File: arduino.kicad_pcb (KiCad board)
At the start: 2 copper layers, 50.8 x 70.6 mm, 30 parts, among them J1 Conn_01x08_Pin, J10 Conn_01x06_Socket, J12 Conn_01x03_Pin, J2 Conn_01x10_Socket, J3 Barrel_Jack_Switch, J4 Conn_01x02_Socket, J5 Conn_01x06_Socket, J8 Conn_01x08_Pin, SW1 SW_Push, U1 ATmega328-P, U2 L7805, U3 LM317_TO-220, Y1 Crystal

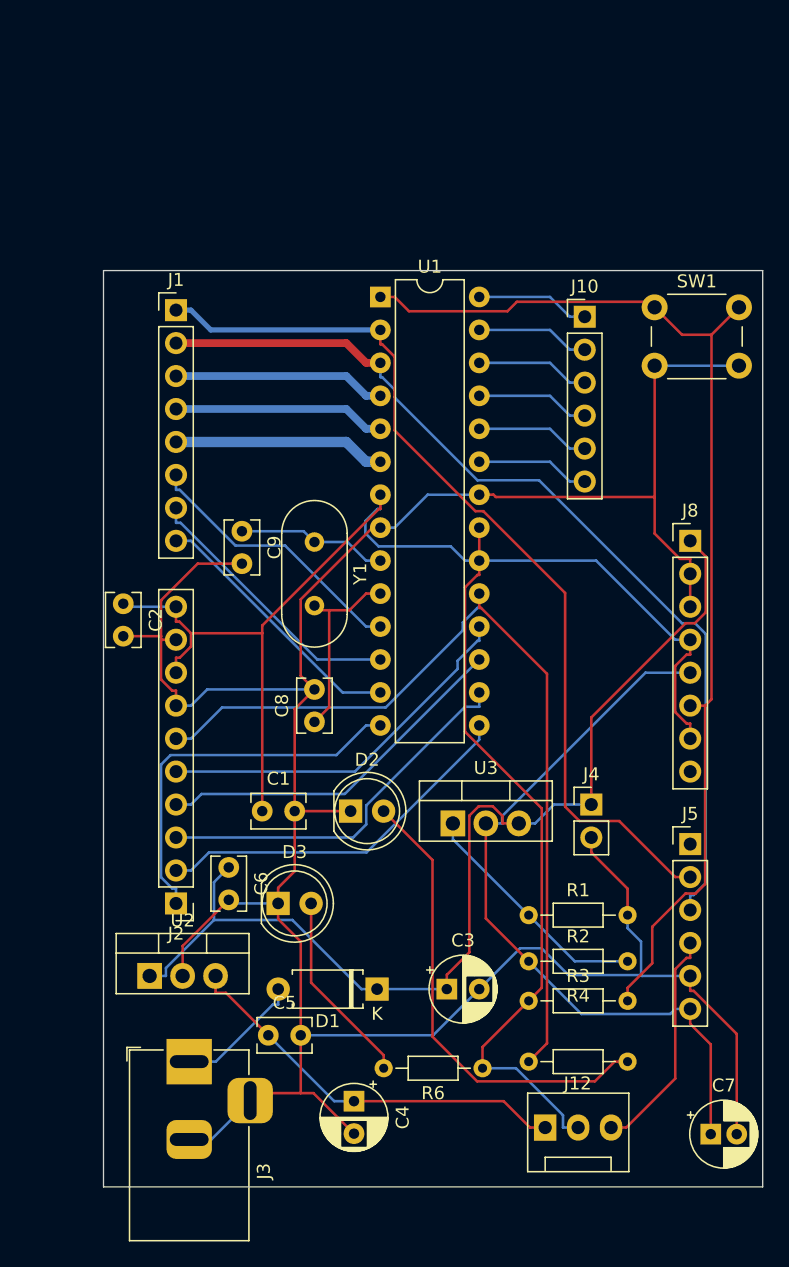
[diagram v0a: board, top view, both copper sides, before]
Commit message: Add files via upload
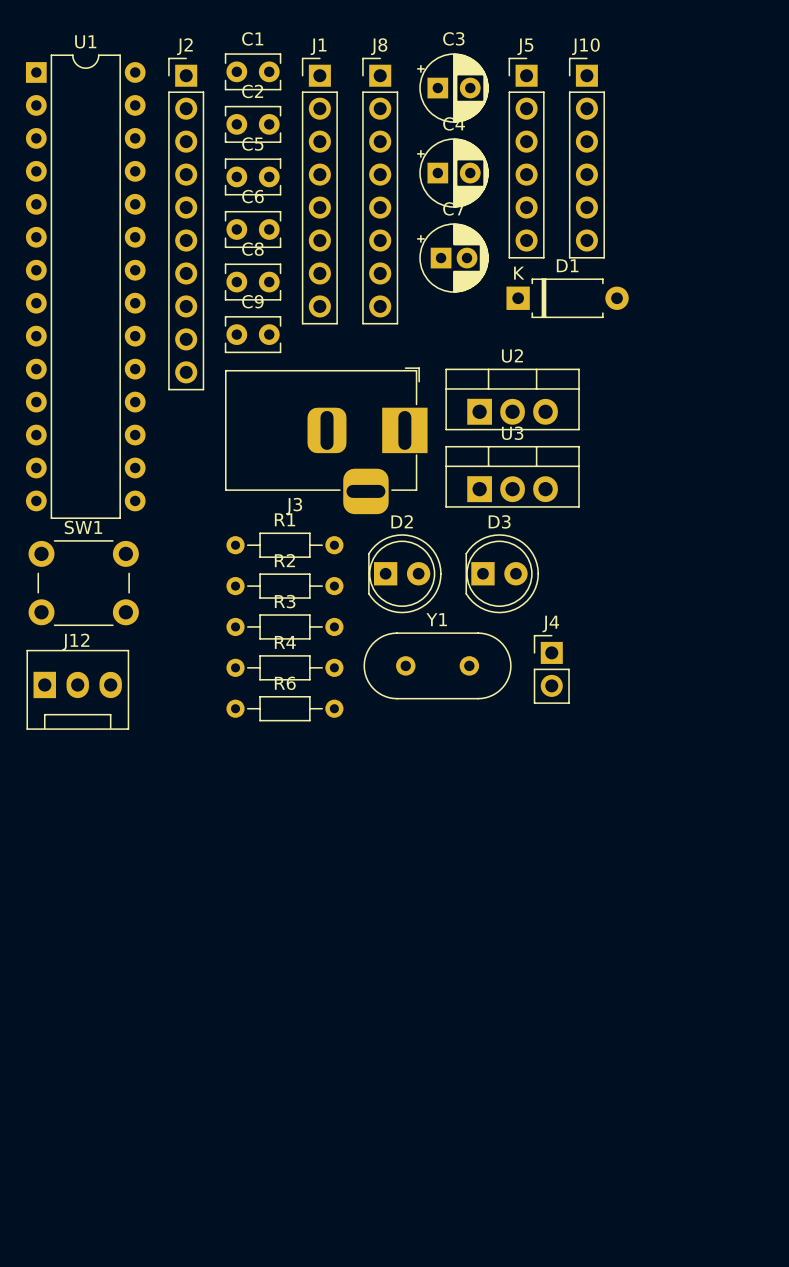
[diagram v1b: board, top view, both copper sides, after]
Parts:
- moved C4 71.8 mm to (233.5, 48.4), turned to 0 degrees
- moved C7 70.6 mm to (233.8, 54.9)
- moved C3 69.4 mm to (233.5, 41.8)
- moved C5 66.2 mm to (218.0, 48.7)
- moved J2 63.8 mm to (214.1, 40.9), turned to 0 degrees
- moved J5 60.5 mm to (240.4, 40.9)
- moved C1 57.0 mm to (218.0, 40.6)
- moved D1 54.3 mm to (239.7, 58.0), turned to 0 degrees
- moved J12 51.5 mm to (203.2, 87.8)
- moved J3 51.4 mm to (231.0, 68.2), turned to 0 degrees
- moved SW1 50.9 mm to (203.0, 77.7)
- moved U2 50.4 mm to (236.8, 66.8)
- moved C6 49.2 mm to (218.0, 52.7), turned to 0 degrees
- moved J8 43.1 mm to (229.1, 40.9)
- moved C2 38.0 mm to (218.0, 44.6), turned to 0 degrees
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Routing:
- net GND: track 219.9 -> 0.00 mm
- net VCC: track 141.5 -> 0.00 mm
- net RST: track 85.9 -> 0.00 mm
- net VIN: track 81.9 -> 0.00 mm
- net TX: track 73.0 -> 0.00 mm
- net RX: track 71.3 -> 0.00 mm
- net D13: track 67.9 -> 0.00 mm
- net 3.3: track 57.5 -> 0.00 mm
- net Net-(D2-A): track 36.0 -> 0.00 mm
- net 5V: track 31.0 -> 0.00 mm
- net D10: track 29.5 -> 0.00 mm
- net D8: track 29.5 -> 0.00 mm
- net D12: track 29.0 -> 0.00 mm
- net D9: track 28.6 -> 0.00 mm
- net D11: track 28.0 -> 0.00 mm
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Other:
- board outline removed
